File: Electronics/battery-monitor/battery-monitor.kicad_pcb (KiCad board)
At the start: 2 copper layers, 2 parts, among them U1 ACS714LLCTR-30A-T, U2 ACS714LLCTR-30A-T

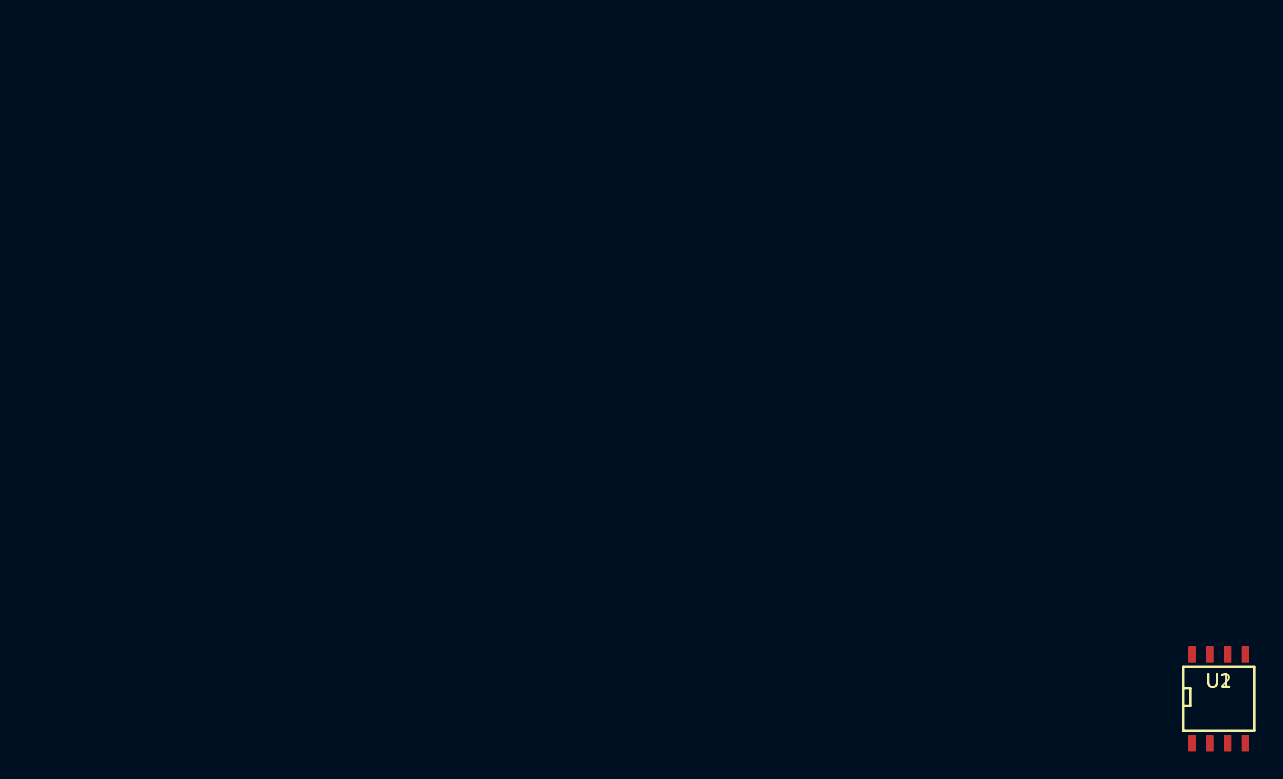
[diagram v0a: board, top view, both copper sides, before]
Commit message: base layout done, freeroute files exported
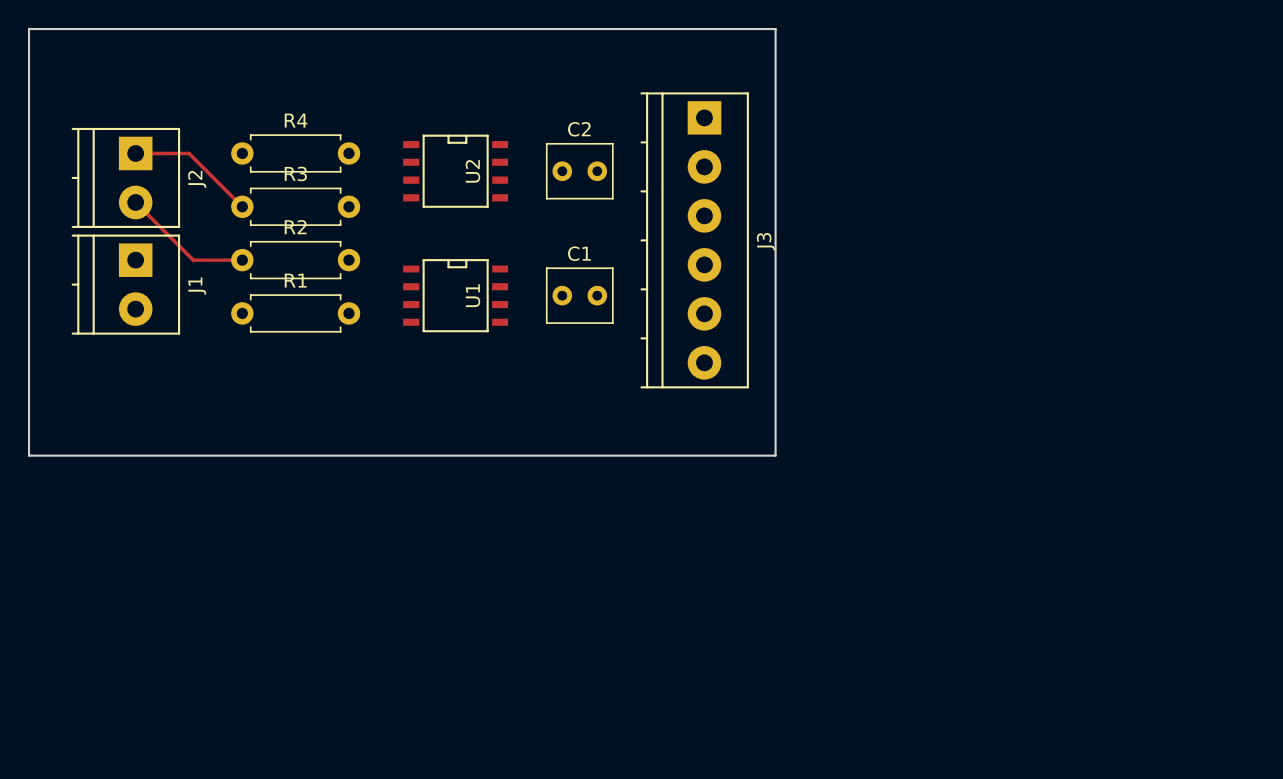
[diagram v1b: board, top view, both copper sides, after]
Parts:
- added C1: C, Capacitors_THT:C_Rect_L4.6mm_W3.8mm_P2.50mm_MKS02_FKP02, F.Cu at (101.6, 76.2)
- added C2: C, Capacitors_THT:C_Rect_L4.6mm_W3.8mm_P2.50mm_MKS02_FKP02, F.Cu at (101.6, 67.3)
- added J1: Screw_Terminal_1x02, Connectors_Terminal_Blocks:TerminalBlock_Pheonix_PT-3.5mm_2pol, F.Cu at (71.1, 73.7)
- added J2: Screw_Terminal_1x02, Connectors_Terminal_Blocks:TerminalBlock_Pheonix_PT-3.5mm_2pol, F.Cu at (71.1, 66.0)
- added J3: Screw_Terminal_1x06, Connectors_Terminal_Blocks:TerminalBlock_Pheonix_PT-3.5mm_6pol, F.Cu at (111.8, 63.5)
- added R1: R, Resistors_THT:R_Axial_DIN0207_L6.3mm_D2.5mm_P7.62mm_Horizontal, F.Cu at (78.7, 77.5)
- added R2: R, Resistors_THT:R_Axial_DIN0207_L6.3mm_D2.5mm_P7.62mm_Horizontal, F.Cu at (78.7, 73.7)
- added R3: R, Resistors_THT:R_Axial_DIN0207_L6.3mm_D2.5mm_P7.62mm_Horizontal, F.Cu at (78.7, 69.8)
- added R4: R, Resistors_THT:R_Axial_DIN0207_L6.3mm_D2.5mm_P7.62mm_Horizontal, F.Cu at (78.7, 66.0)
- moved U2 66.3 mm to (94.0, 67.3), turned to 270 degrees
- moved U1 61.7 mm to (94.0, 76.2), turned to 270 degrees
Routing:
- net GND: track 0.00 -> 9.33 mm
- net Net-(J2-Pad1): track 0.00 -> 9.20 mm
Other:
- board outline added: 53.3 x 30.5 mm
